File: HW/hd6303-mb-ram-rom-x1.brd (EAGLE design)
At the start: 100 x 80 mm, 33 parts, among them IC2 AM29F010N

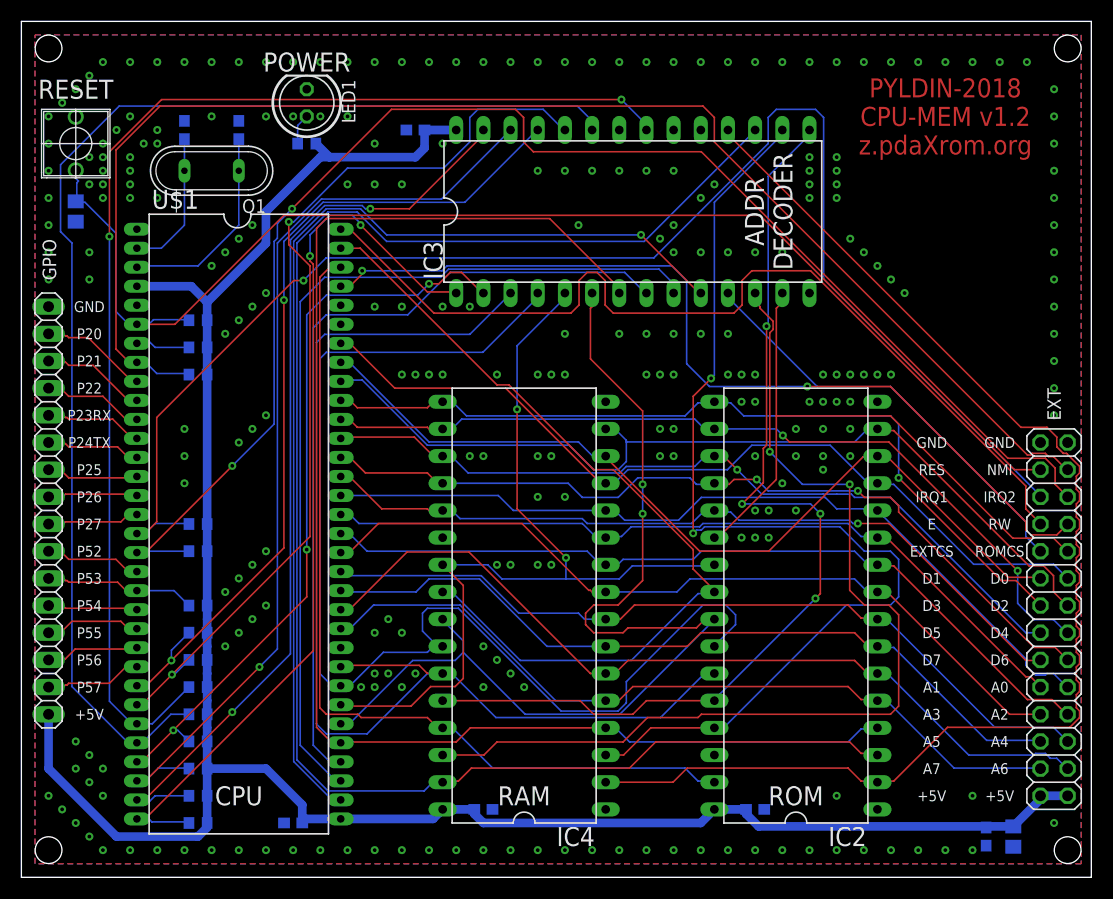
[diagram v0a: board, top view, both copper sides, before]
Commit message: released in pcb
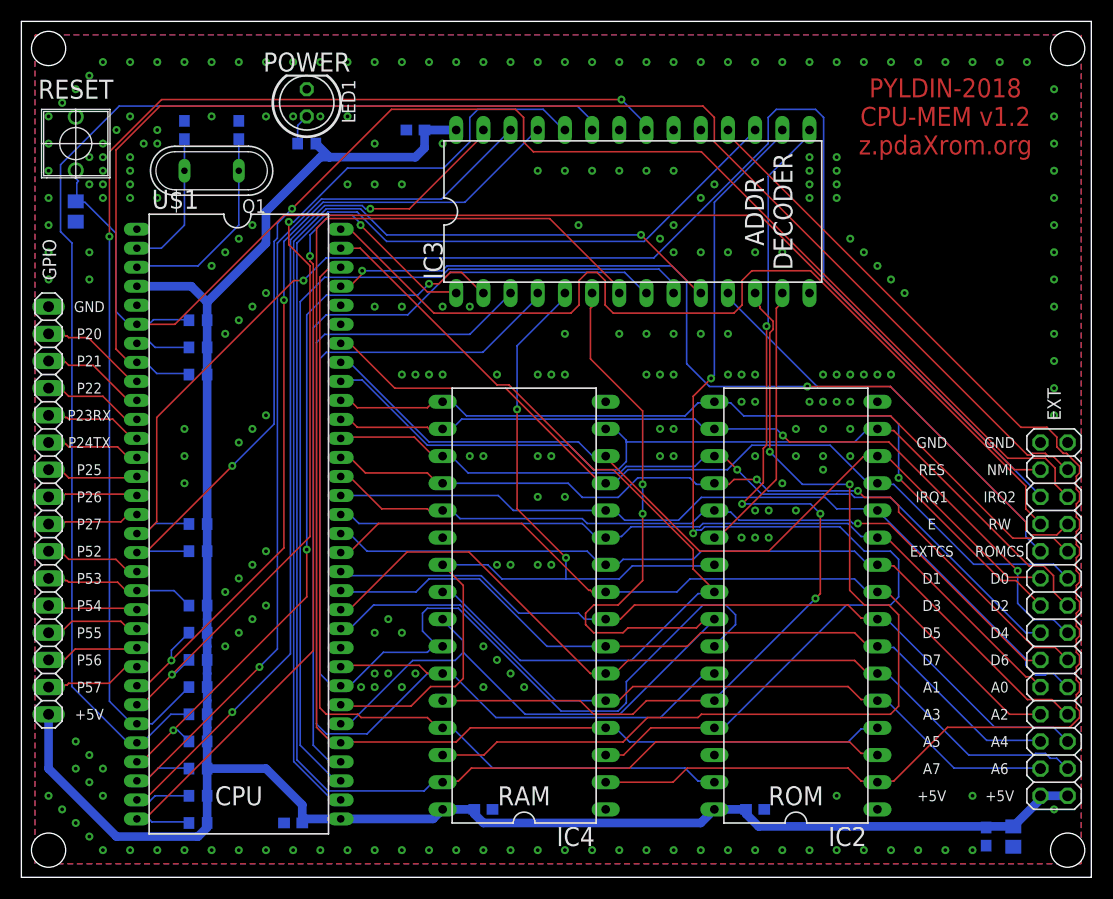
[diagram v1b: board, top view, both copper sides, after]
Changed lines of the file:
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@@
 <wire x1="100" y1="80" x2="0" y2="80" width="0" layer="20"/>
 <wire x1="0" y1="80" x2="0" y2="0" width="0" layer="20"/>
-<hole x="2.54" y="77.47" drill="2.5"/>
-<hole x="2.54" y="2.54" drill="2.5"/>
-<hole x="97.79" y="2.54" drill="2.5"/>
-<hole x="97.79" y="77.47" drill="2.5"/>
-<text x="86.36" y="71.12" size="1.778" layer="1" font="vector" align="center">PYLDIN-2018
+<hole x="2.54" y="77.47" drill="3.2" locked="yes"/>
+<hole x="2.54" y="2.54" drill="3.2" locked="yes"/>
+<hole x="97.79" y="2.54" drill="3.2" locked="yes"/>
+<hole x="97.79" y="77.47" drill="3.2" locked="yes"/>
+<text x="86.36" y="71.12" locked="yes" size="1.778" layer="1" font="vector" align="center">PYLDIN-2018
 CPU-MEM v1.2
 z.pdaXrom.org</text>
@@
 <attribute name="VALUE" x="73.279" y="8.509" size="1.778" layer="27" rot="R90"/>
 </element>
-<element name="EXT" library="pinhead" library_urn="urn:adsk.eagle:library:325" package="2X14" package3d_urn="urn:adsk.eagle:package:22426/2" value="" x="96.52" y="24.13" smashed="yes" rot="R270">
+<element name="EXT" library="pinhead" library_urn="urn:adsk.eagle:library:325" package="2X14" package3d_urn="urn:adsk.eagle:package:22426/2" value="" x="96.52" y="24.13" locked="yes" smashed="yes" rot="R270">
 <attribute name="NAME" x="95.885" y="45.72" size="1.27" layer="25" ratio="10" rot="R270"/>
 <attribute name="VALUE" x="92.075" y="41.91" size="1.27" layer="27" rot="R270"/>
@@
 <attribute name="VALUE" x="13.335" y="9.525" size="1.27" layer="28" rot="MR180"/>
 </element>
-<element name="GPIO" library="pinhead" library_urn="urn:adsk.eagle:library:325" package="1X16" package3d_urn="urn:adsk.eagle:package:22432/2" value="" x="2.54" y="34.29" smashed="yes" rot="R270">
+<element name="GPIO" library="pinhead" library_urn="urn:adsk.eagle:library:325" package="1X16" package3d_urn="urn:adsk.eagle:package:22432/2" value="" x="2.54" y="34.29" locked="yes" smashed="yes" rot="R270">
 <attribute name="NAME" x="3.2512" y="55.8038" size="1.27" layer="25" ratio="10" rot="R90"/>
 <attribute name="VALUE" x="-0.635" y="54.61" size="1.27" layer="27" rot="R270"/>
@@
 <via x="21.59" y="53.34" extent="1-16" drill="0.35"/>
 <via x="22.86" y="54.61" extent="1-16" drill="0.35"/>
-<via x="96.52" y="5.08" extent="1-16" drill="0.35"/>
+<via x="96.52" y="6.35" extent="1-16" drill="0.35"/>
 <via x="88.9" y="7.62" extent="1-16" drill="0.35"/>
 <via x="88.9" y="2.54" extent="1-16" drill="0.35"/>
@@
 packages will not be understood (or retained) with this version.
 </note>
+<note version="8.5" severity="warning">
+Since Version 8.5, EAGLE supports locking for holes, vias, wires and polygons.
+The locking property on all objects of these types will not be understood in this version.
+</note>
 </compatibility>
